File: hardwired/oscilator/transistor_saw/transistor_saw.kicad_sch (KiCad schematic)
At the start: 21 parts, among them Q1 PNP, Q2 NPN, U1 ${SIM.PARAMS}, U2 ${SIM.PARAMS}

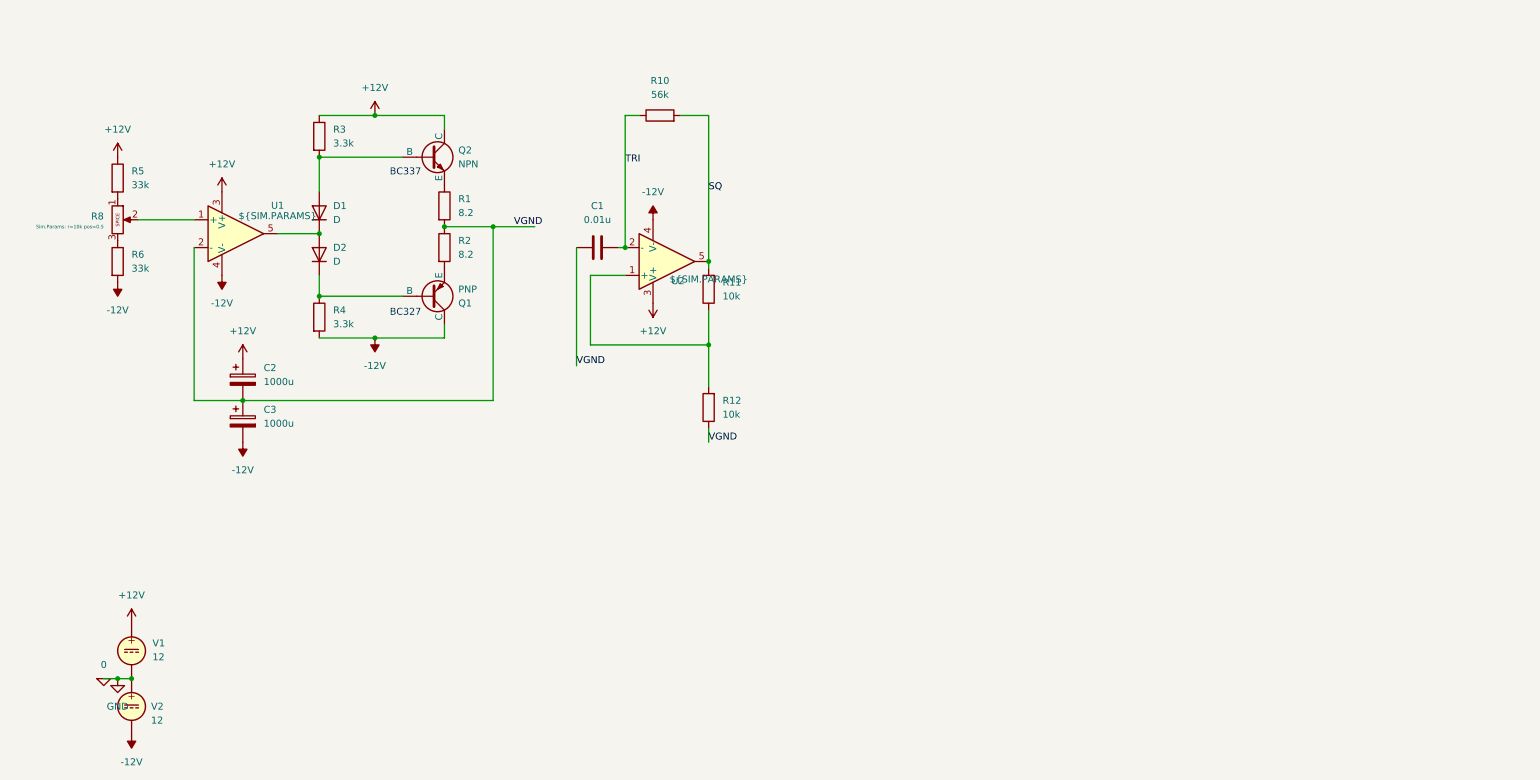
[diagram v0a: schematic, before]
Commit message: Massive dump of circuits and code
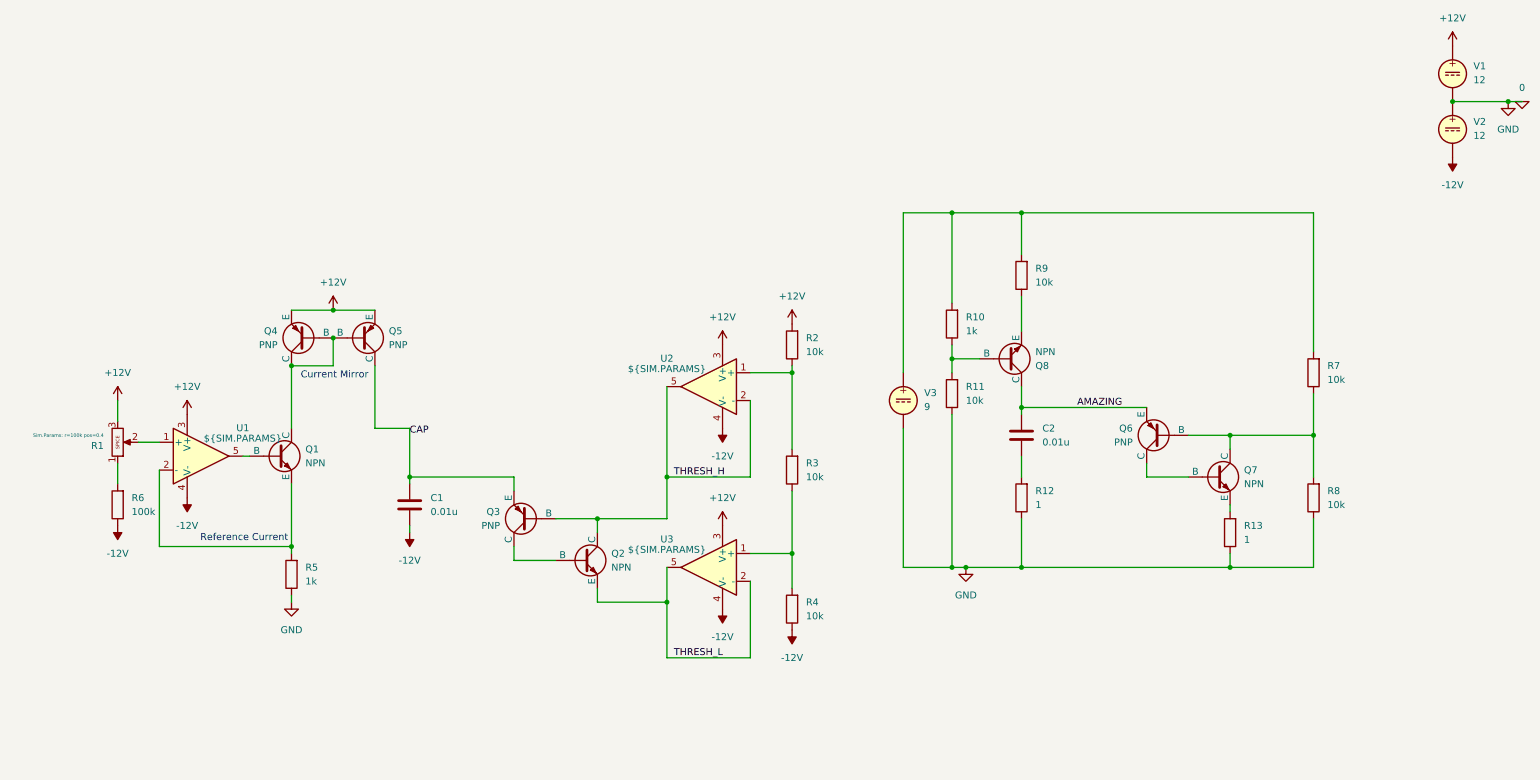
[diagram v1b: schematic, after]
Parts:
- removed C2, C3: 1000u, Connector_PinSocket_2.54mm:PinSocket_1x02_P2.54mm_Vertical, symbol Device:C_Polarized
- removed D1, D2: D, Diode_THT:D_A-405_P7.62mm_Horizontal, symbol Device:D
- removed Q1: PNP, Connector_PinSocket_2.54mm:PinSocket_1x03_P2.54mm_Vertical, symbol Simulation_SPICE:PNP
- removed R1: 8.2, Resistor_THT:R_Axial_DIN0309_L9.0mm_D3.2mm_P15.24mm_Horizontal, symbol Device:R
- removed R8: Potentiometer, Connector_PinHeader_2.54mm:PinHeader_1x03_P2.54mm_Horizontal, symbol Simulation_SPICE:Potentiometer
- added C2: 0.01u, symbol Device:C
- added Q1, Q7, Q8: NPN, symbol Simulation_SPICE:NPN
- added Q3, Q4, Q5, Q6: PNP, symbol Simulation_SPICE:PNP
- added R1: Potentiometer, symbol Simulation_SPICE:Potentiometer
- added R13: 1, symbol Device:R
- added R7, R8, R9: 10k, symbol Device:R
- added U3: ${SIM.PARAMS}, symbol Simulation_SPICE:OPAMP
- added V3: 9, symbol Simulation_SPICE:VDC
- Q2: footprint Connector_PinSocket_2.54mm:PinSocket_1x03_P2.54mm_Vertical -> (none)
- R10: value 56k -> 1k; footprint Resistor_THT:R_Axial_DIN0411_L9.9mm_D3.6mm_P15.24mm_Horizontal -> (none)
- R11: footprint Resistor_THT:R_Axial_DIN0411_L9.9mm_D3.6mm_P15.24mm_Horizontal -> (none)
- R12: value 10k -> 1; footprint Resistor_THT:R_Axial_DIN0411_L9.9mm_D3.6mm_P15.24mm_Horizontal -> (none)
- R2: value 8.2 -> 10k; footprint Resistor_THT:R_Axial_DIN0309_L9.0mm_D3.2mm_P15.24mm_Horizontal -> (none)
- R3, R4: value 3.3k -> 10k; footprint Resistor_THT:R_Axial_DIN0309_L9.0mm_D3.2mm_P15.24mm_Horizontal -> (none)
- R5: value 33k -> 1k; footprint Resistor_THT:R_Axial_DIN0309_L9.0mm_D3.2mm_P15.24mm_Horizontal -> (none)
- R6: value 33k -> 100k; footprint Resistor_THT:R_Axial_DIN0309_L9.0mm_D3.2mm_P15.24mm_Horizontal -> (none)
- U1, U2: footprint Package_DIP:DIP-8_W7.62mm -> (none)
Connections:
- net +12V: now also R2.2, Q4.3 (E), Q5.3 (E), R1.3, U3.3 (V+); no longer Q2.1 (C), R3.1, R5.1
- net -12V: now also C1.2, R4.1, R6.1, U3.4 (V-); no longer R4.2, R6.2
- net 0: now also R11.1, R12.1, R5.1, R13.1, R8.1, V3.2
- net at U1.1 (+): now also R1.2
- net at U1.5: now also Q1.2 (B)
- net at R3.2: now also R2.1, U2.1 (+); no longer Q2.2 (B)
- net THRESH_L: now reaches Q2.3 (E)
- net THRESH_L: now also U3.2 (-), U3.5
- net at R5.2: now also U1.2 (-), Q1.3 (E)
- removed net SQ: R10.2, R11.2, U2.5
- removed net TRI: C1.2, R10.1, U2.2 (-)
- removed net VGND: C1.1, R12.1, R2.1, U1.2 (-)
- new net: Q8.2 (B), R10.1, R11.2
- new net: Q2.2 (B), Q3.1 (C)
- new net: Q8.3 (E), R9.1
- new net: Q6.2 (B), Q7.1 (C), R7.1, R8.2
- new net: R10.2, R7.2, R9.2, V3.1
- new net: Q1.1 (C), Q4.1 (C), Q4.2 (B), Q5.2 (B)
- new net: R1.1, R6.2
- new net: C2.2, R12.2
- new net: R3.1, R4.2, U3.1 (+)
- new net: Q7.3 (E), R13.2
- new net: Q6.1 (C), Q7.2 (B)
- new net AMAZING: C2.1, Q6.3 (E), Q8.1 (C)
- new net CAP: C1.1, Q3.3 (E), Q5.1 (C)
- new net THRESH_H: Q2.1 (C), Q3.2 (B), U2.2 (-), U2.5
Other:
- note added: "Current Mirror"
- note added: "Reference Current"
- note removed: "BC327"
- note removed: "BC337"
